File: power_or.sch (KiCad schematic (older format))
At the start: 48 parts

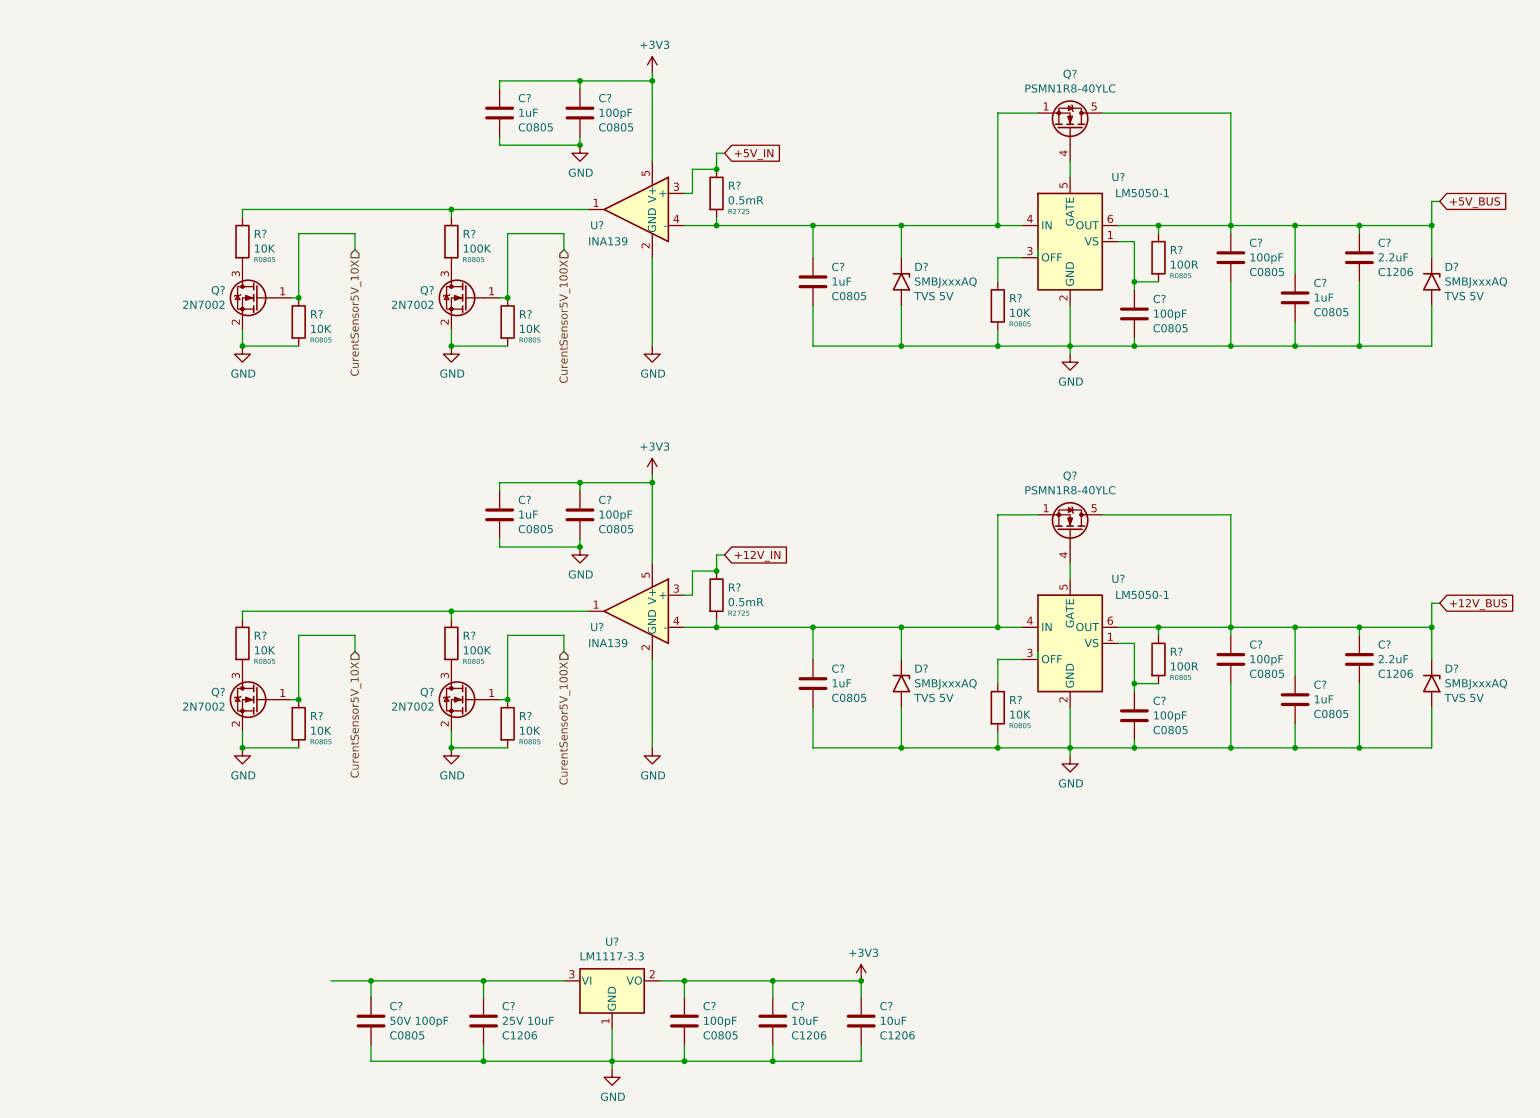
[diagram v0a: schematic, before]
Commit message: power or switch v1
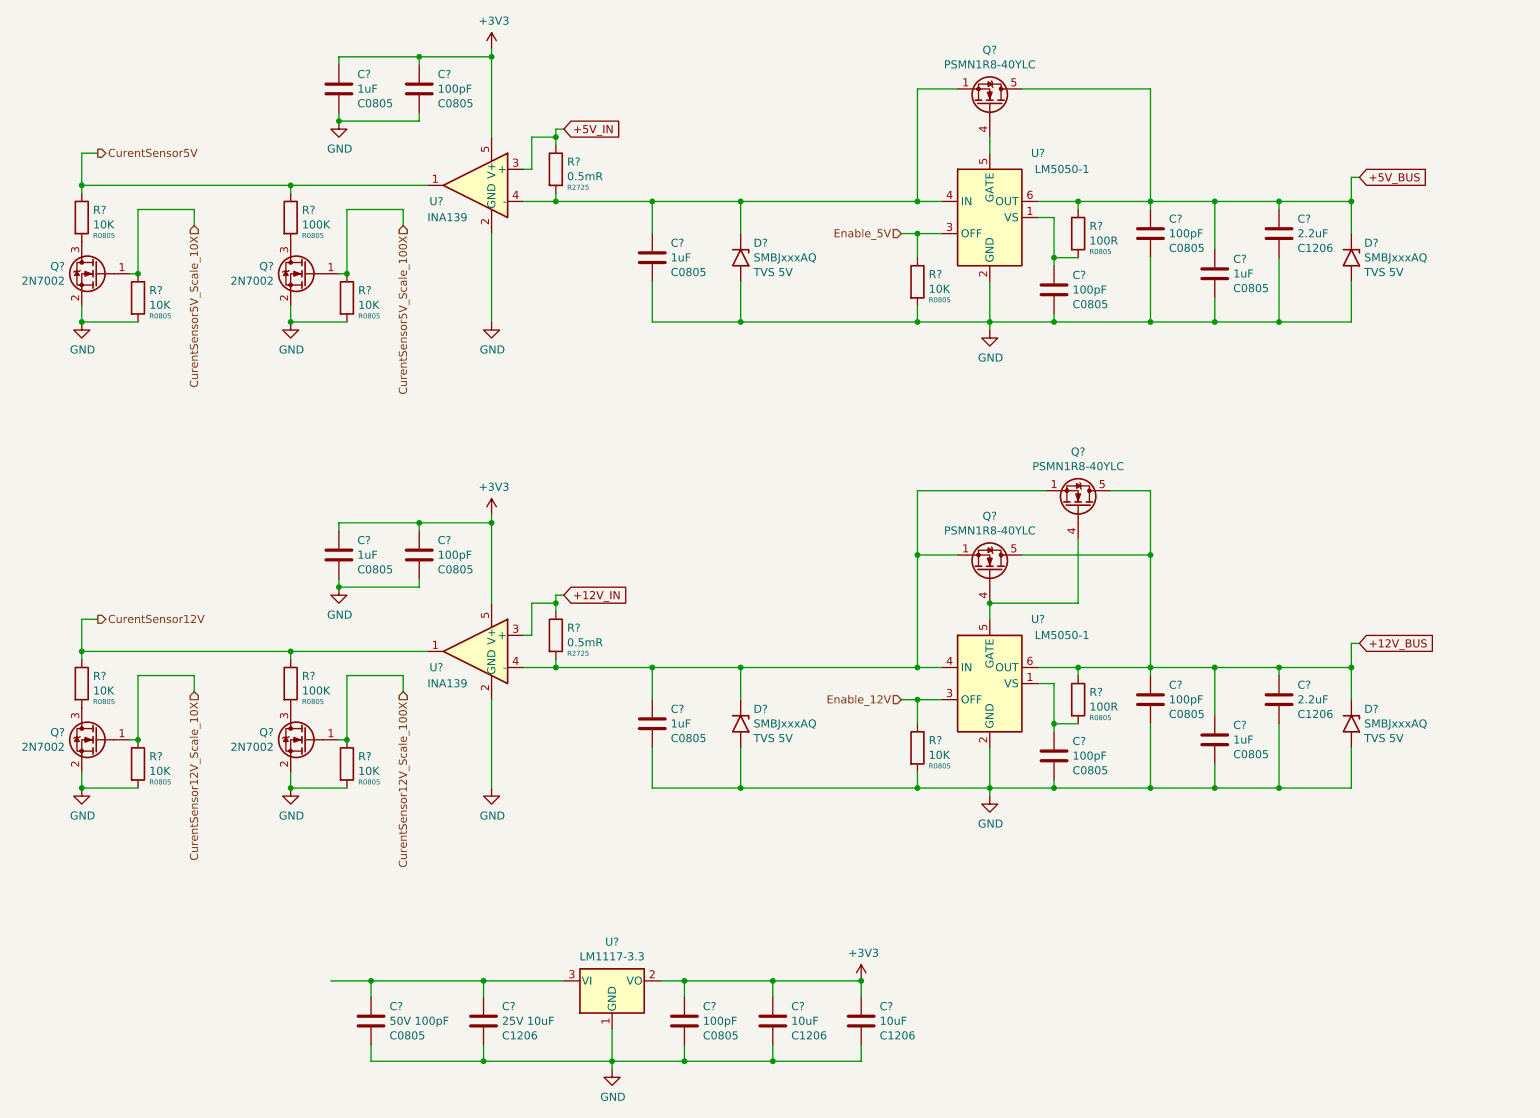
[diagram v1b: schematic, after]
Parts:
- added Q?: PSMN1R8-40YLC, Package_TO_SOT_SMD:LFPAK56, symbol Transistor_FET:PSMN1R8-40YLC
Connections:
- net labels added: CurentSensor12V, CurentSensor12V_Scale_100X, CurentSensor12V_Scale_10X, CurentSensor5V, CurentSensor5V_Scale_100X, CurentSensor5V_Scale_10X, Enable_12V, Enable_5V
- net labels removed: CurentSensor5V_100X, CurentSensor5V_10X
- wire segments 185 -> 197
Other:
- moved on the sheet: C?, D?, Q?, R?, U?
